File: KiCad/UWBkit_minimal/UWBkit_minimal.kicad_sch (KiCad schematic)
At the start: 56 parts, among them J1 Conn_UART, J2 Conn_SWD, J3 USB_C_Receptacle_USB2.0_14P, J4 Conn_BATT, J5 Jumper_Cell_NO, Q1 BSS138, Q2 BSS138, Q3 BSS341, SW1 SW_Push, U1 DWM3001C, U2 IP4234CZ6, U3 MAX40203AUK+T, U4 XC9285B33CMR-G

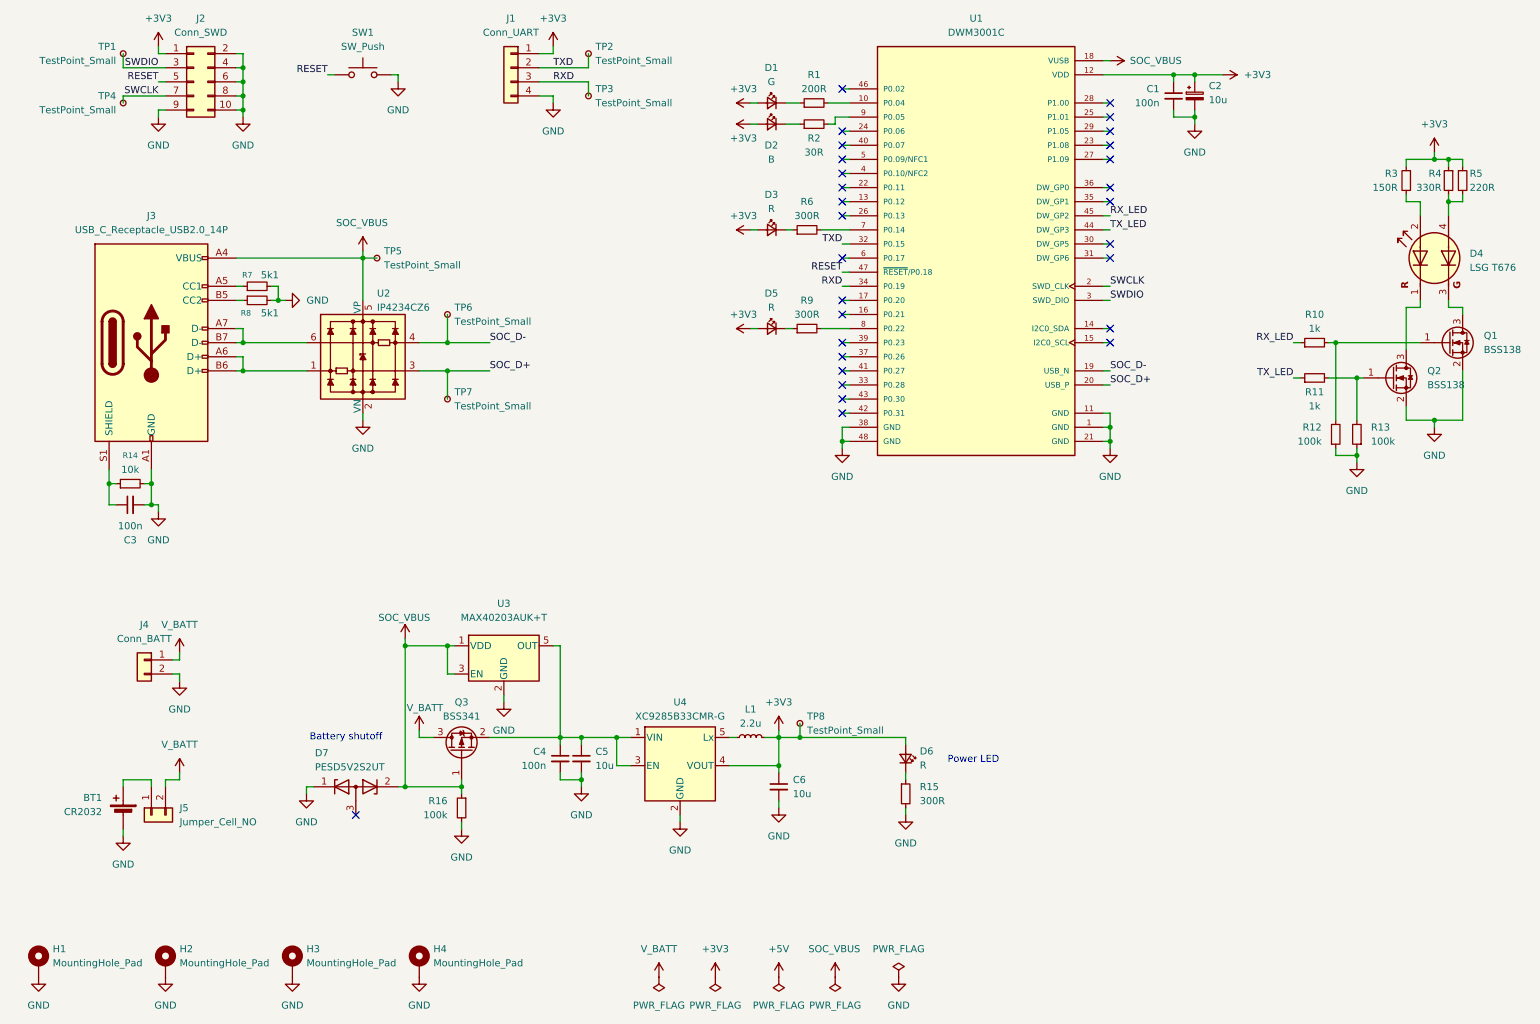
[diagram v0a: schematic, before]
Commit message: Generated BOM
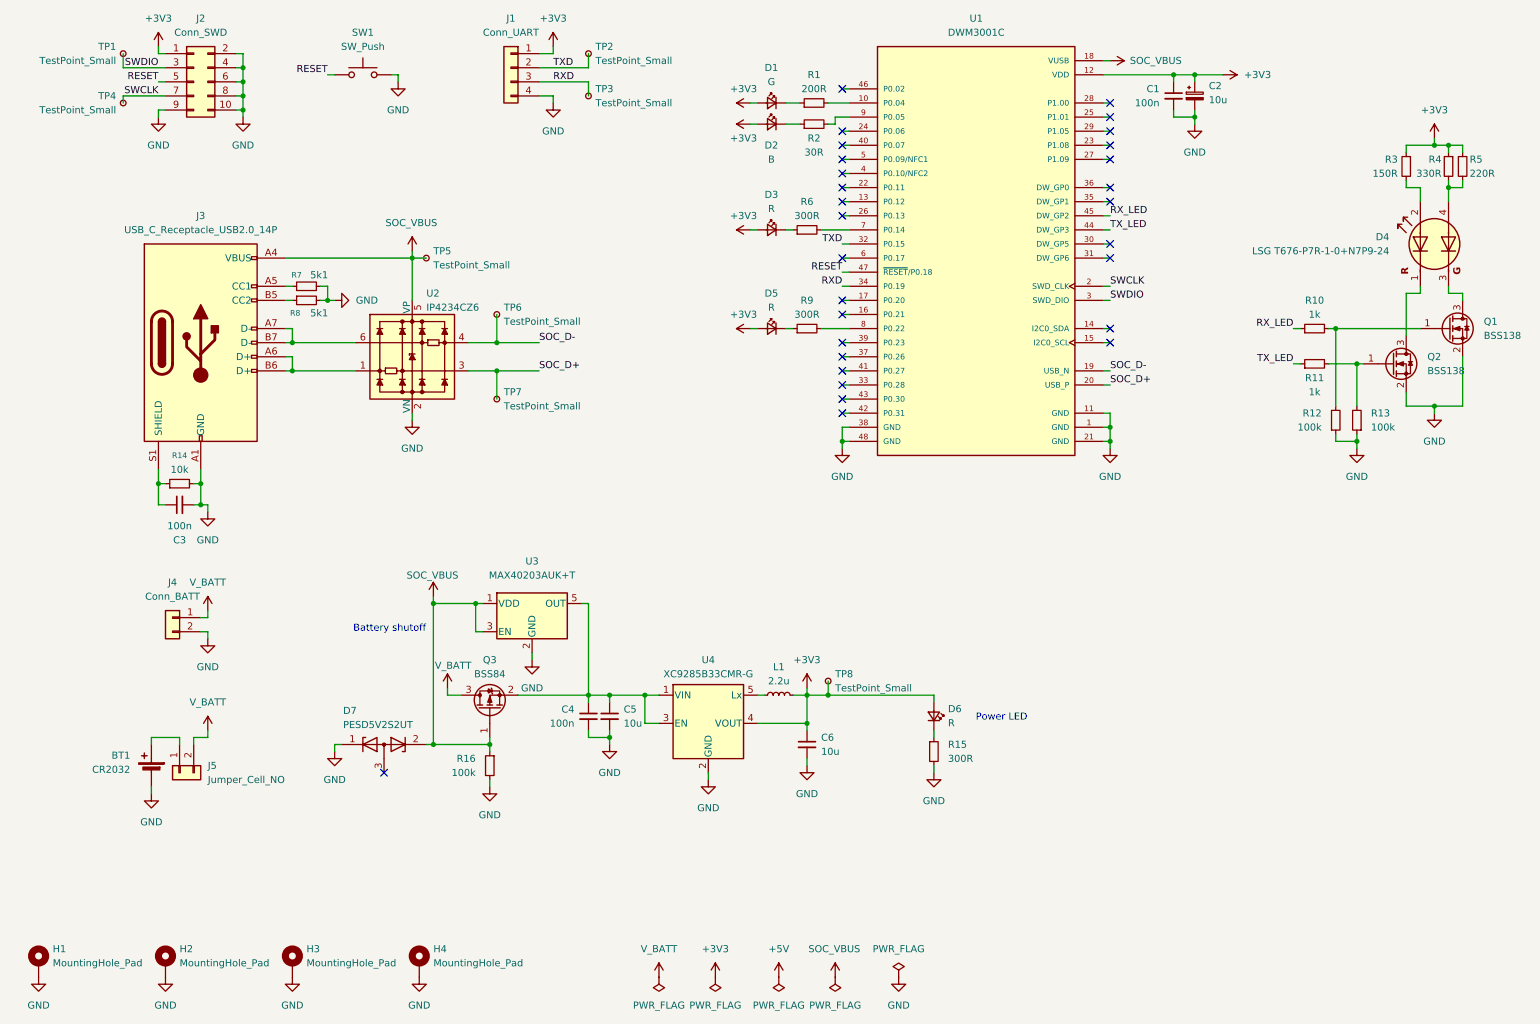
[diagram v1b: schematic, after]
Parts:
- D4: value LSG T676 -> LSG T676-P7R-1-0+N7P9-24
- Q3: value BSS341 -> BSS84
- TP1, TP2, TP3, TP4, TP5, TP6, TP7, TP8: now left out of the parts list
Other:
- moved on the sheet: BT1, C3, C4, C5, C6, D4, D6, D7, J3, J4, J5, L1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
